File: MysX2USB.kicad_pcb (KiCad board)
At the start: 2 copper layers, 13.4 x 17.6 mm, 9 parts, among them P1 USB, P2 MYSX_1.2, P3 supply, U1 FT230XS

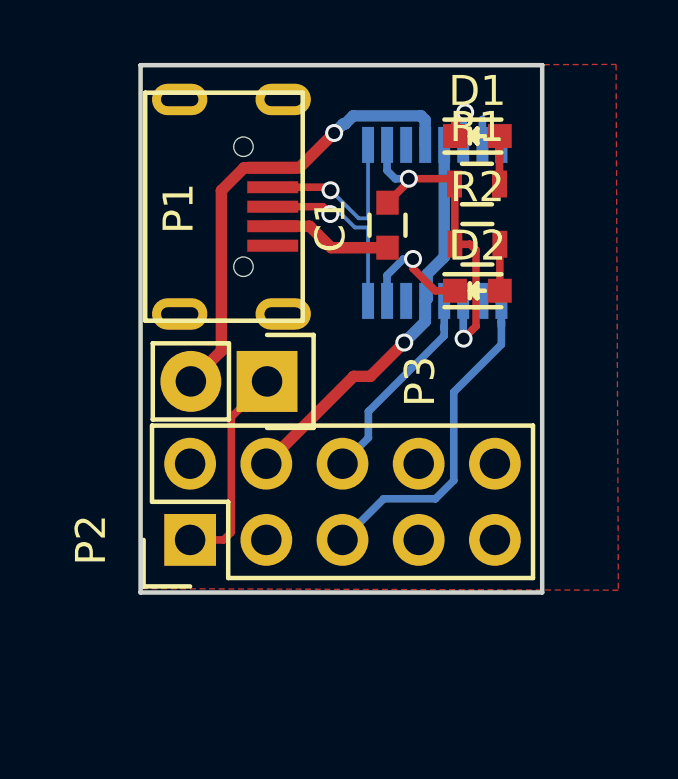
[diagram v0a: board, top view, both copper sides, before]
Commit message: Updated to MysX2.0
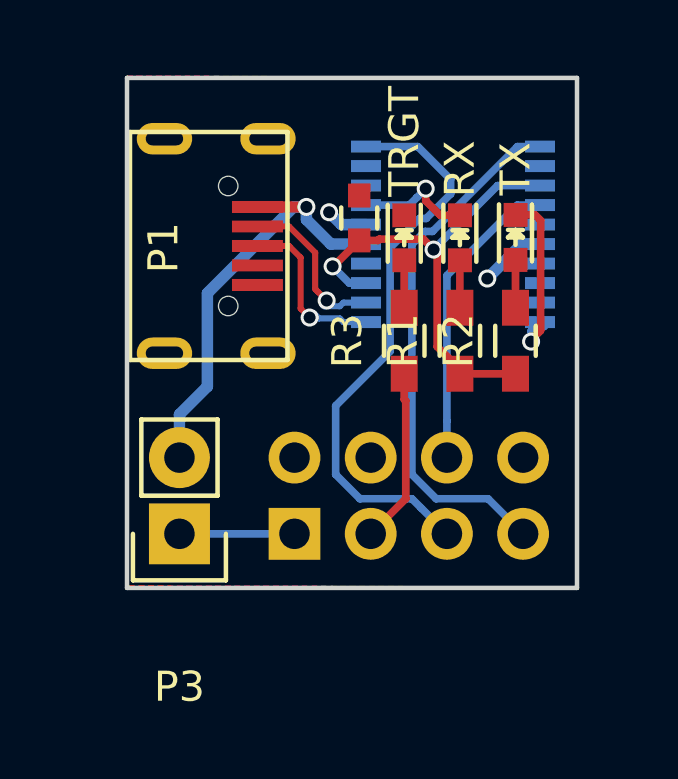
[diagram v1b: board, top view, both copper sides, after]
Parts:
- added D3: TRGT, LEDs:LED-0603, F.Cu at (123.2, 115.3)
- added R3: R, Resistors_SMD:R_0603_HandSoldering, F.Cu at (123.2, 118.8)
- D1: value LED -> RX
- D2: value LED -> TX
- P1: value USB -> USB_A
- P2: value MYSX_1.2 -> MYSX_2.0; footprint mysensors_connectors:MYSX_1.1 -> mysensors_connectors:MYSX_2.0_SOCKET
- R1, R2: footprint Resistors_SMD:R_0603 -> Resistors_SMD:R_0603_HandSoldering
- U1: value FT230XS -> FT231XS; footprint Housings_SSOP:SSOP-16_3.9x4.9mm_Pitch0.635mm -> Housings_SSOP:SSOP-20_4.4x6.5mm_Pitch0.65mm
- moved P3 5.86 mm to (115.7, 125.2), turned to 180 degrees
- moved R1 5.26 mm to (125.1, 118.8), turned to 90 degrees
- moved P2 3.49 mm to (119.6, 125.2)
- moved R2 3.46 mm to (126.9, 118.8), turned to 90 degrees
- moved D1 3.44 mm to (125.1, 115.3), turned to 270 degrees
- moved D2 2.18 mm to (126.9, 115.3), turned to 270 degrees
- moved P1 1.40 mm to (114.1, 115.6)
- moved C1 0.97 mm to (121.7, 114.7), turned to 270 degrees
- moved U1 0.72 mm to (124.9, 115.2), turned to 180 degrees
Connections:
- P2 pad 7: Net-(P2-Pad7) -> /RST
- U1 pad 1: /TXD -> /RST
- U1 pad 10: Net-(C1-Pad2) -> Net-(D2-Pad1)
- U1 pad 11: Net-(U1-Pad11) -> /D+
- U1 pad 12: +5V -> /D-
- U1 pad 13: GND -> Net-(C1-Pad2)
- U1 pad 14: Net-(D1-Pad1) -> Net-(U1-Pad14)
- U1 pad 15: Net-(U1-Pad15) -> +5V
- U1 pad 16: Net-(U1-Pad16) -> GND
- U1 pad 5: GND -> Net-(U1-Pad5)
- U1 pad 6: Net-(U1-Pad6) -> GND
- U1 pad 7: Net-(D2-Pad1) -> Net-(U1-Pad7)
- U1 pad 8: /D+ -> Net-(U1-Pad8)
- U1 pad 9: /D- -> Net-(U1-Pad9)
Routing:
- net /RST: track 0.00 -> 17.8 mm
- net GND: track 17.5 -> 3.63 mm, vias 1 -> 2
- net /TXD: track 11.4 -> 19.4 mm
- net Net-(P2-Pad3): track 0.00 -> 5.84 mm
- net Net-(C1-Pad2): track 11.6 -> 16.0 mm
- net /RXD: track 6.93 -> 10.1 mm
- net Net-(P2-Pad1): track 7.00 -> 3.84 mm
- net Net-(D2-Pad1): track 3.97 -> 6.07 mm
- net Net-(D1-Pad1): track 2.25 -> 3.96 mm
- net Net-(D3-Pad2): track 0.00 -> 1.58 mm
- net Net-(U1-Pad15): track 0.85 -> 0.00 mm
- net /D-: track 6.59 -> 5.76 mm
- net +5V: track 15.5 -> 14.7 mm
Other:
- board size 13.4 x 17.6 mm -> 15 x 17 mm
